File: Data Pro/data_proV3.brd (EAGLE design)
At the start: 100 x 80 mm, 47 parts, among them IC1 4049N, IC2 MCP3008, IC3 OP11S, IC4 LM340MP-05, IC6 AT24CP, J1 RASPBERRYPI-40-PIN-GPIO, U1 DS18B20, X1 32.768khz

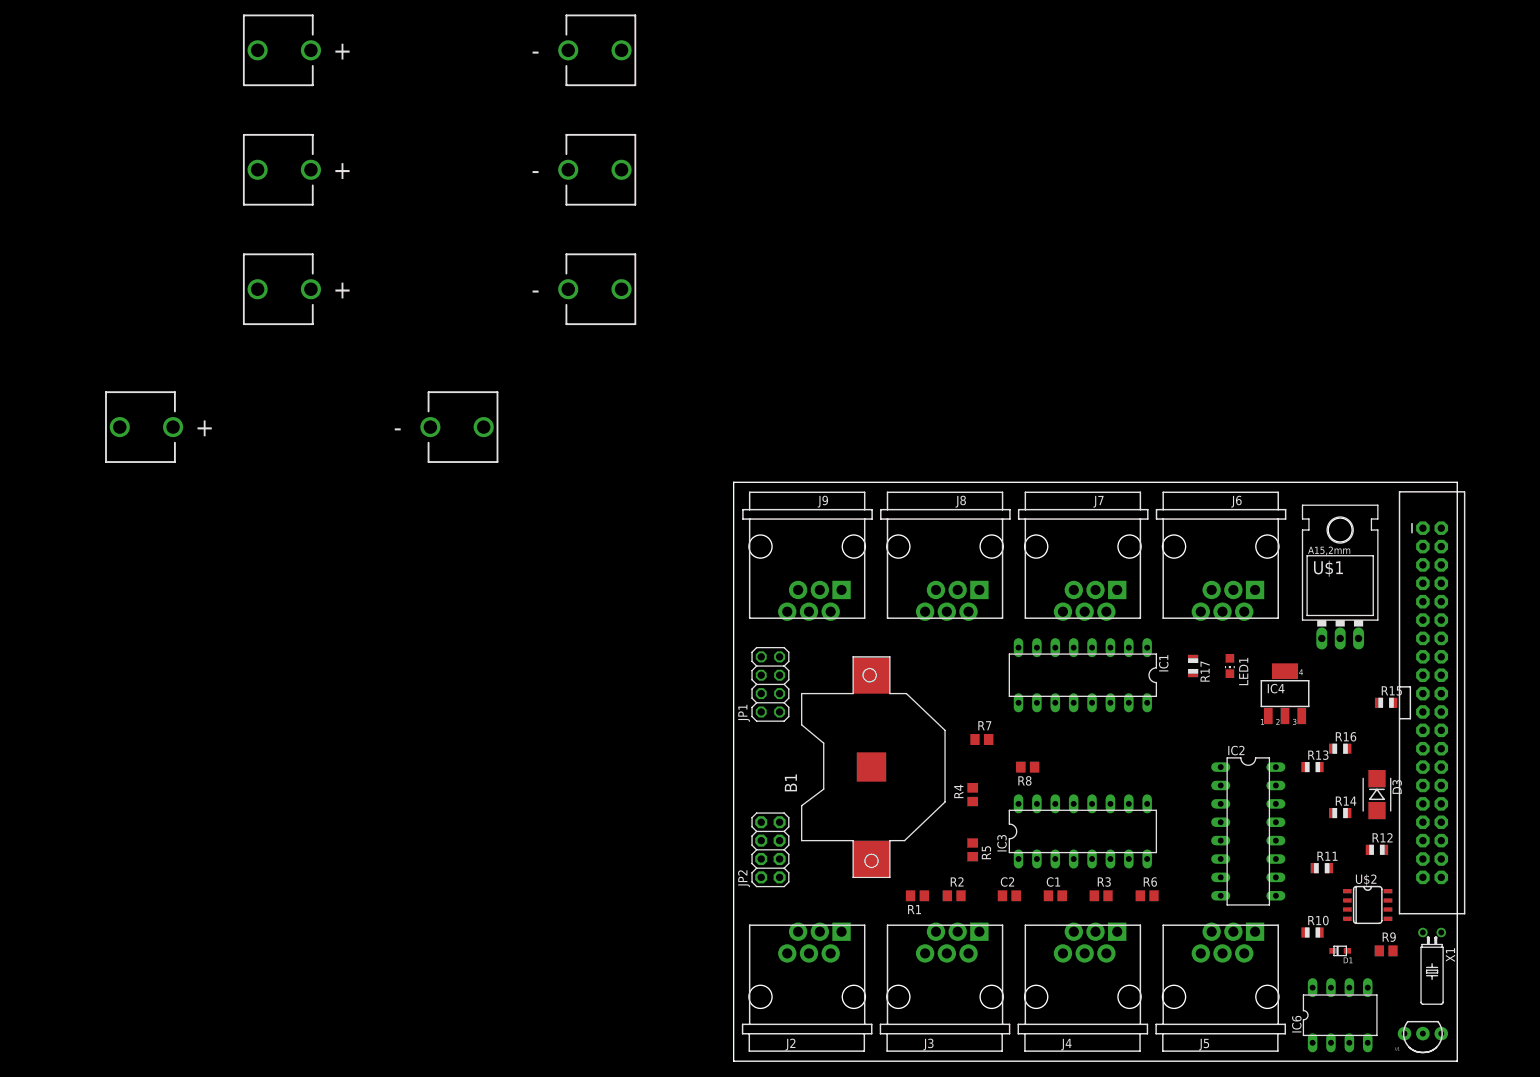
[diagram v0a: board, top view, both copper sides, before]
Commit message: Data pro update and Lewis' python code
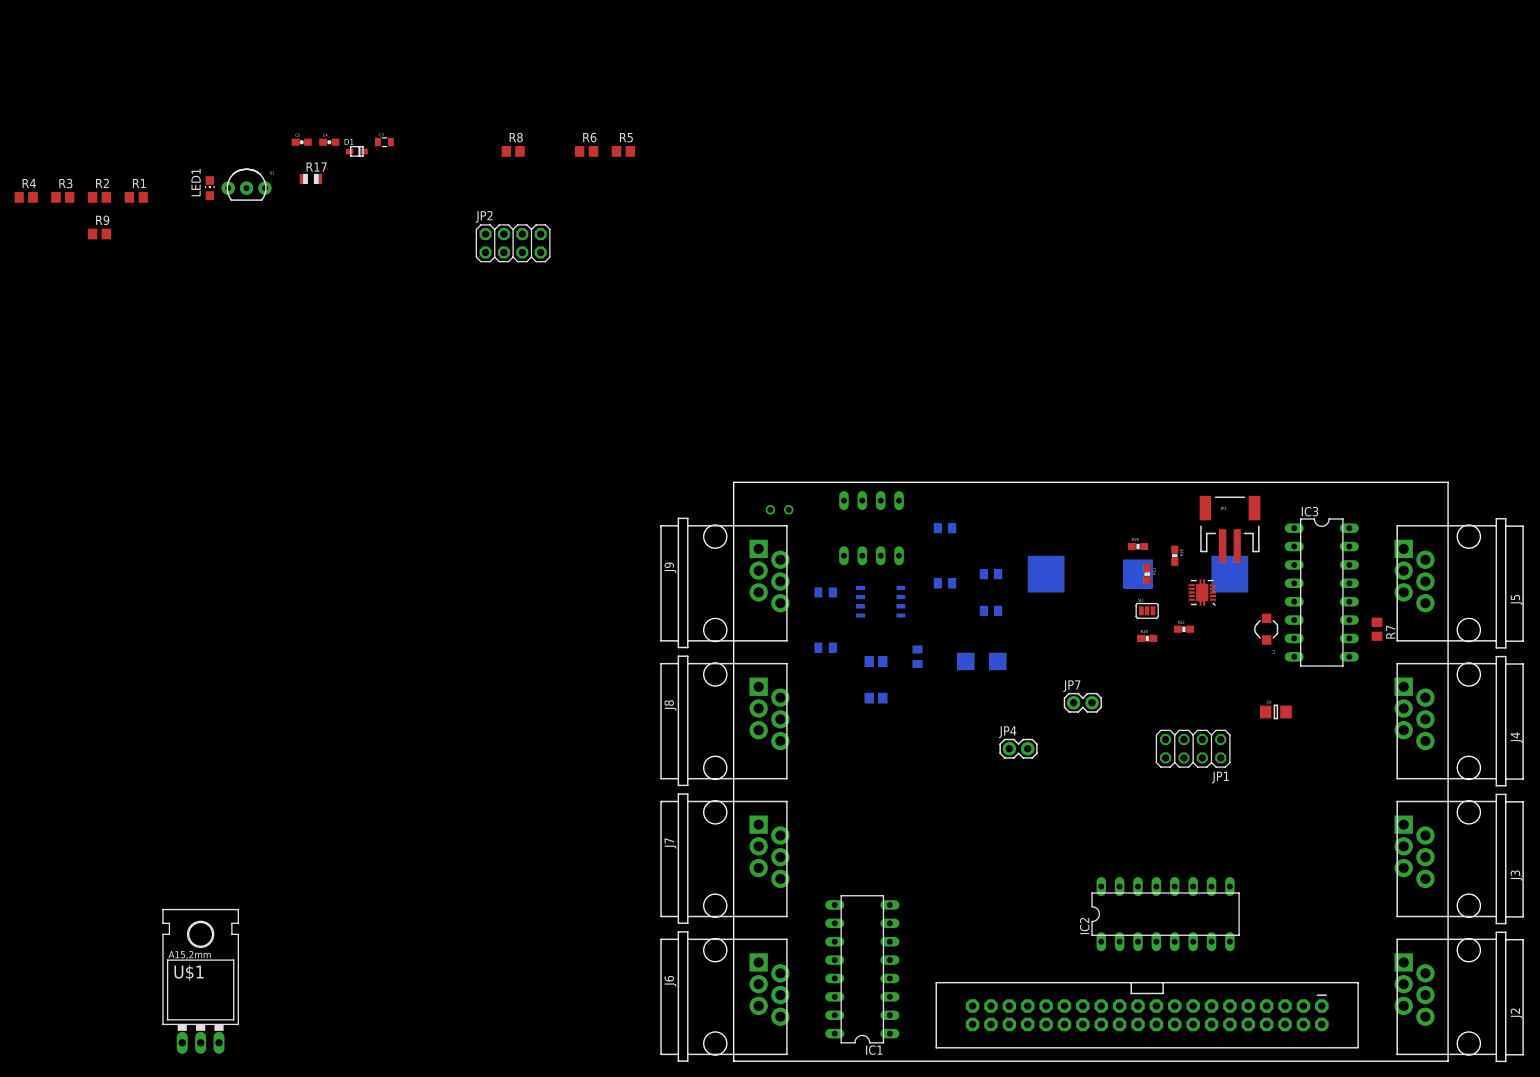
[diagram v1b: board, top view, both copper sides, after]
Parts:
- removed BAT1, BAT2, BAT3, BAT4: (no value), SparkFun-Electromechanical:BATTERY-AA
- removed IC4: LM340MP-05, linear:SOT223
- added C3: 22uF, CH_passive:0805
- added C4, C5: 0.1uF, SparkFun:0603-CAP
- added C6: 10uF, CH_passive:1206
- added JP3: JST, SparkFun:JST-2-SMD
- added JP4: VOUT, SparkFun:1X02
- added JP7: VIN, SparkFun:1X02
- added L1: 4.7uH, 1.2A, SparkFun:CDRH2D09
- added R18, R22: 2M, SparkFun:0603-RES
- added R19, R21: 220k, SparkFun:0603-RES
- added R20: 1.2M, SparkFun:0603-RES
- added SJ1: (no value), SparkFun:SJ_3_PASTE2&3
- added U2: TPS61200, SparkFun:QFN-10_PAD
- B1: value (none) -> CR2032
- moved R9 203.5 mm to (-87.6, 114.3)
- moved U1 200.2 mm to (-67.3, 120.7), turned to 0 degrees
- moved D1 175.1 mm to (-52.1, 125.7), turned to 0 degrees
- moved R3 172.9 mm to (-92.7, 119.4)
- moved U$1 167.1 mm to (-73.7, 6.35)
- moved LED1 155.7 mm to (-72.4, 120.7), turned to 0 degrees
- moved R4 154.7 mm to (-97.8, 119.4), turned to 0 degrees
- moved R2 152.5 mm to (-87.6, 119.4)
- moved R1 144.8 mm to (-82.5, 119.4), turned to 0 degrees
- moved R17 139.3 mm to (-58.4, 121.9), turned to 0 degrees
- moved R6 128.8 mm to (-20.3, 125.7)
- moved R8 110.9 mm to (-30.5, 125.7), turned to 0 degrees
- moved R5 107.9 mm to (-15.2, 125.7), turned to 0 degrees
- moved X1 107.4 mm to (6.35, 76.2), flipped to the bottom
- moved J6 93.5 mm to (-2.54, 8.89), turned to 270 degrees
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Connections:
- removed net GPIO0: JP2.6
- removed net GPIO2: JP2.4
- removed net IRQ: JP1.8
- removed net N$21: IC1.4
- removed net N$22: IC1.6
- removed net N$23: IC1.10
- removed net RST: JP2.5
- removed net S1-10V: J2.6, J3.6, J4.6, J5.6
- new net D1: IC1.2, J1.29
- new net D2: IC1.4, J1.31
- new net D3: IC1.6, J1.32
- new net D4: IC1.10, J1.33
- new net FB: R21.2, SJ1.2, U2.10
- new net UVLO: C4.2, R18.1, R19.2, U2.7
- new net VIN: C4.1, C6.1, JP3.2, JP7.2, L1.P$2, R18.2, U2.5, U2.6, U2.8
- net 3.3V: now also IC6.8, JP2.5, R20.1, SJ1.1
- net 5V: now also R22.1, SJ1.3; no longer IC4.3
- net GND: now also C3.2, C5.2, C6.2, JP3.1, JP4.1, JP7.1, R19.1, R21.1, U2.11, U2.12, U2.13, U2.14, U2.15, U2.4, U2.9; no longer BAT1.PWR@1, BAT2.PWR@1, BAT3.PWR@1, BAT4.PWR@1, IC4.4
- net N$13: now also C5.1, U2.1; no longer IC1.2
- net N$9: now also L1.P$1, U2.3; no longer BAT1.GND@1, BAT2.GND@1, BAT3.GND@1, BAT4.GND@1, IC4.1
- net VCC: now also C3.1, JP4.2, R20.2, R22.2, U2.2; no longer IC6.8
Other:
- board size 100 x 80 mm -> 98.7 x 80 mm
